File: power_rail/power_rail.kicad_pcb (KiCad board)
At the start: 2 copper layers, 100 x 50 mm, 18 parts, among them J1 Conn_01x06, J2 Conn_02x08_Row_Letter_Last, J3 Conn_02x08_Row_Letter_Last, J4 Conn_02x08_Row_Letter_Last, J5 Conn_02x08_Row_Letter_Last, J6 Conn_02x08_Row_Letter_Last, J7 Conn_02x08_Row_Letter_Last, J8 Conn_01x06

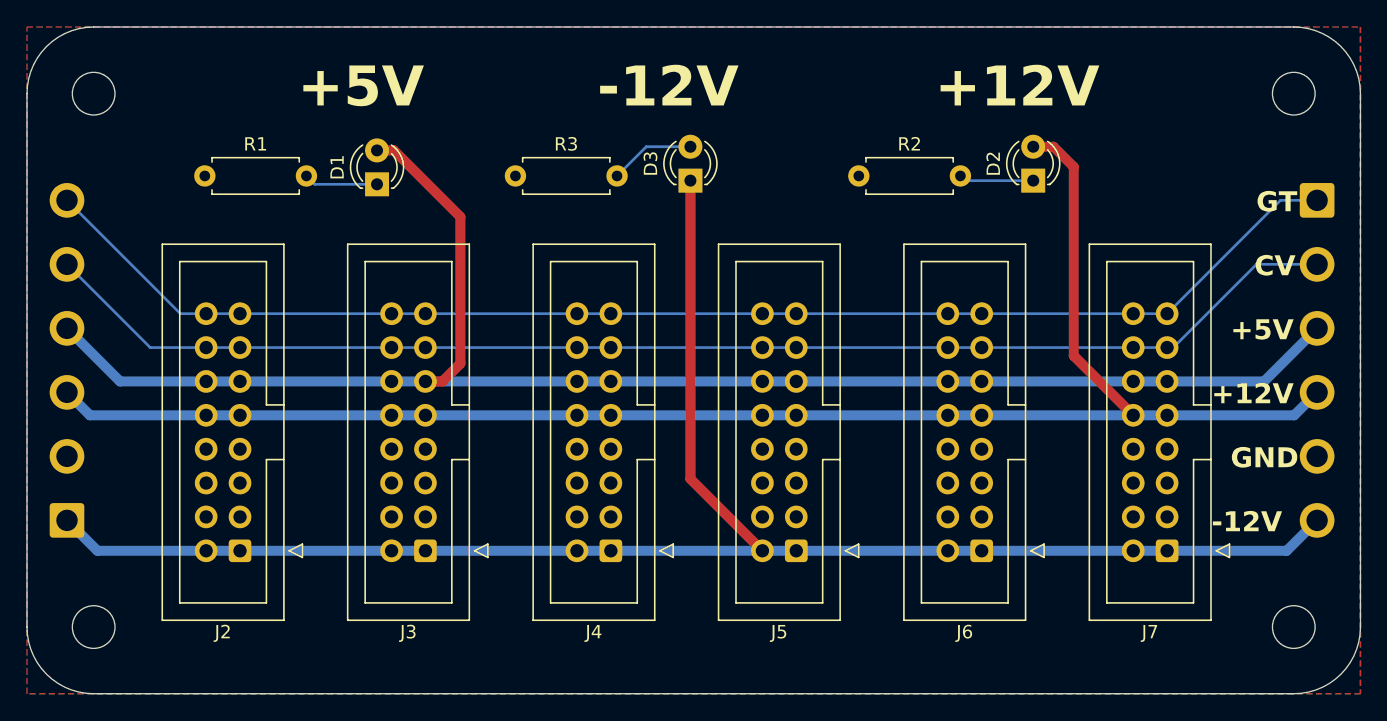
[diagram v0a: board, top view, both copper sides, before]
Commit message: VCA v. 2.0
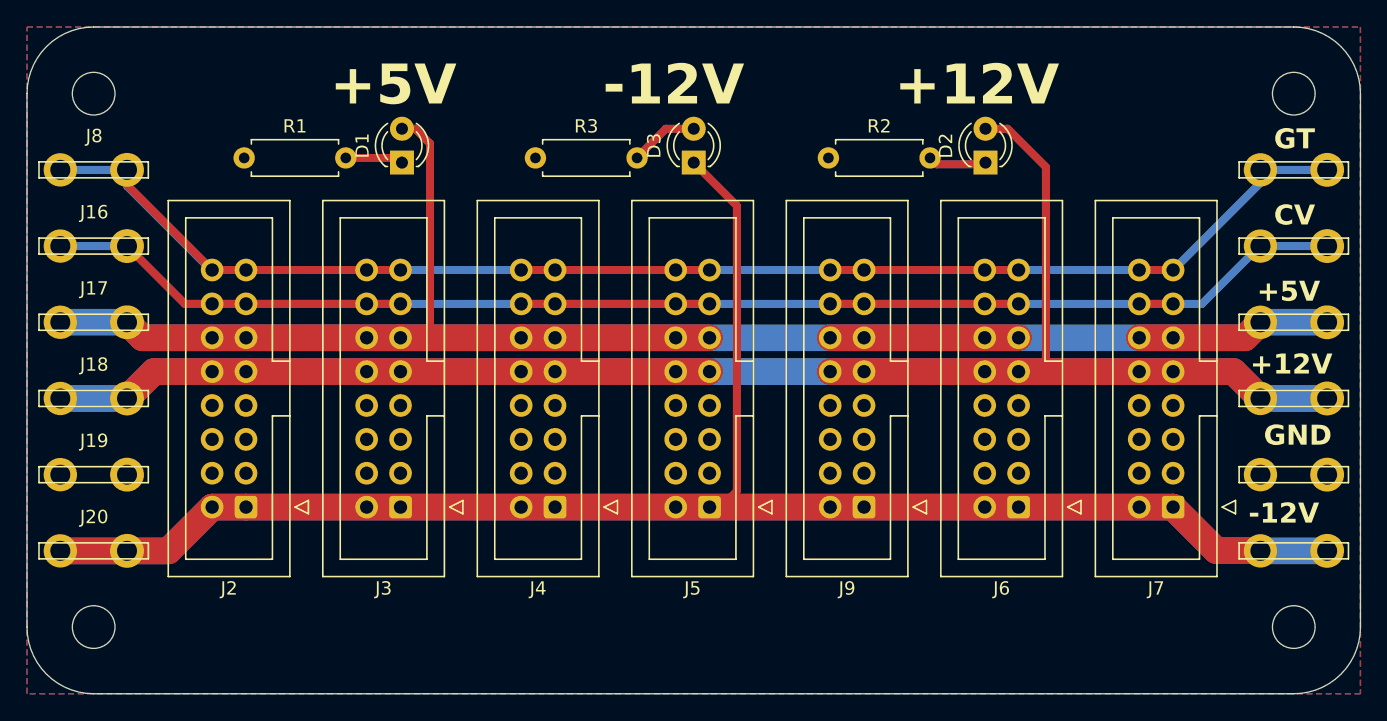
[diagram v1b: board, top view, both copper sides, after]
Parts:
- added J11: Conn_01x01_Pin, power_rail_elements:Blade_3866B.68, F.Cu at (197.5, 96.4)
- added J12: Conn_01x01_Pin, power_rail_elements:Blade_3866B.68, F.Cu at (197.5, 102.1)
- added J13: Conn_01x01_Pin, power_rail_elements:Blade_3866B.68, F.Cu at (197.5, 107.9)
- added J14: Conn_01x01_Pin, power_rail_elements:Blade_3866B.68, F.Cu at (197.5, 113.6)
- added J15: Conn_01x01_Pin, power_rail_elements:Blade_3866B.68, F.Cu at (197.5, 119.3)
- added J16: Conn_01x01_Pin, power_rail_elements:Blade_3866B.68, F.Cu at (107.5, 96.4)
- added J17: Conn_01x01_Pin, power_rail_elements:Blade_3866B.68, F.Cu at (107.5, 102.1)
- added J18: Conn_01x01_Pin, power_rail_elements:Blade_3866B.68, F.Cu at (107.5, 107.9)
- added J19: Conn_01x01_Pin, power_rail_elements:Blade_3866B.68, F.Cu at (107.5, 113.6)
- added J20: Conn_01x01_Pin, power_rail_elements:Blade_3866B.68, F.Cu at (107.5, 119.3)
- added J9: Conn_02x08_Row_Letter_Last, Connector_IDC:IDC-Header_2x08_P2.54mm_Vertical, F.Cu at (167.8, 116.0)
- J1, J8: value Conn_01x06 -> Conn_01x01_Pin; footprint Connector_Wire:SolderWire-0.75sqmm_1x06_P4.8mm_D1.25mm_OD2.3mm -> power_rail_elements:Blade_3866B.68
- moved J8 94.3 mm to (107.5, 90.7), turned to 0 degrees
- moved J1 93.3 mm to (197.5, 90.7), turned to 0 degrees
- moved J5 7.28 mm to (156.2, 116.0)
- moved J4 5.32 mm to (144.6, 116.0)
- moved J6 4.29 mm to (179.4, 116.0)
- moved D2 3.83 mm to (176.9, 90.2)
- moved J3 3.77 mm to (133.0, 116.0)
- moved J2 3.31 mm to (121.4, 116.0)
- moved J7 3.31 mm to (190.9, 116.0)
- moved R1 3.24 mm to (121.3, 89.8)
- moved R2 2.65 mm to (165.1, 89.8)
- moved D1 2.48 mm to (133.1, 90.2)
- moved R3 2.02 mm to (143.1, 89.8)
- moved D3 1.37 mm to (155.0, 90.2)
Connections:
- J1 pad 1: /-12V -> /Gate
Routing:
- net /-12V: track 125.6 -> 219.0 mm
- net /+12V: track 119.3 -> 194.5 mm
- net /+5V: track 119.5 -> 179.9 mm
- net /Gate: track 100.8 -> 157.6 mm
- net /CV: track 98.9 -> 151.7 mm
- net Net-(D3-A): track 6.41 -> 5.18 mm
- net Net-(D2-K): track 5.60 -> 4.41 mm
- net Net-(D1-K): track 5.55 -> 4.36 mm
